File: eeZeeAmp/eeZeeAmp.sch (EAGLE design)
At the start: 11 parts, among them IC1 LM386

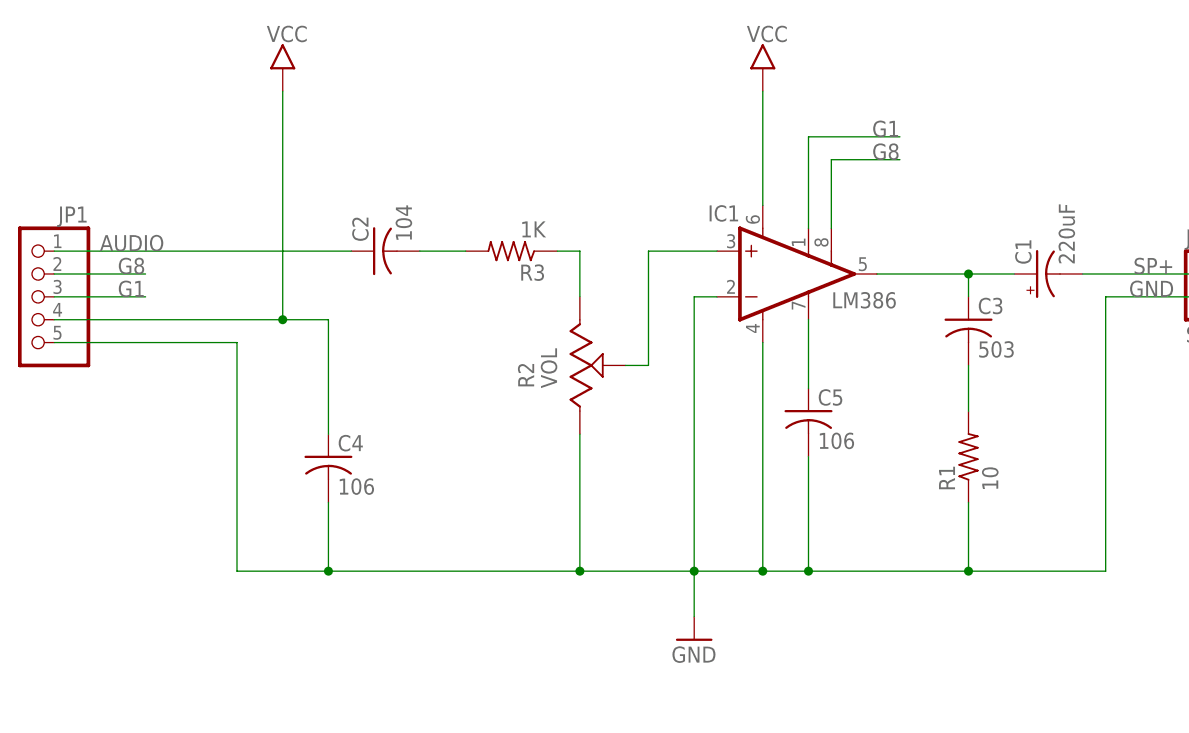
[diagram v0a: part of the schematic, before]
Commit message: Minor updates, added gerbers, zip
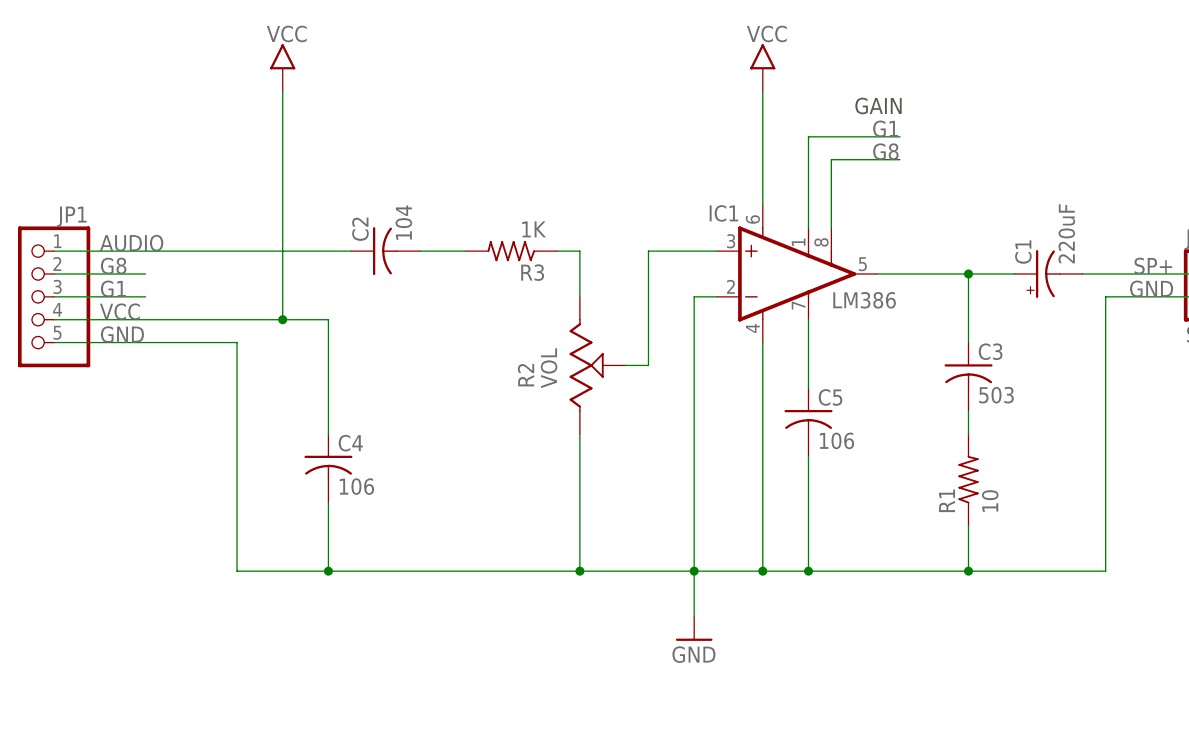
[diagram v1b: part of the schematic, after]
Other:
- note added: "GAIN"
- moved on the sheet: C3, R1
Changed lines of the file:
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@@
 <text x="159.258" y="24.13" size="3.81" layer="94">eeZeeAmp</text>
 <text x="231.14" y="24.13" size="3.81" layer="94">R0.1</text>
+<text x="142.24" y="129.54" size="1.778" layer="97">GAIN</text>
 </plain>
 <instances>
@@
 <instance part="C1" gate="G$1" x="162.56" y="111.76" rot="R90"/>
 <instance part="C2" gate="G$1" x="88.9" y="114.3" rot="R90"/>
-<instance part="C3" gate="G$1" x="154.94" y="106.68"/>
-<instance part="R1" gate="G$1" x="154.94" y="91.44" rot="R90"/>
+<instance part="C3" gate="G$1" x="154.94" y="101.6"/>
+<instance part="R1" gate="G$1" x="154.94" y="88.9" rot="R90"/>
 <instance part="R2" gate="1" x="111.76" y="101.6"/>
 <instance part="JP2" gate="A" x="185.42" y="109.22"/>
@@
 <pinref part="C3" gate="G$1" pin="1"/>
 <wire x1="160.02" y1="111.76" x2="154.94" y2="111.76" width="0.1524" layer="91"/>
-<wire x1="154.94" y1="111.76" x2="154.94" y2="109.22" width="0.1524" layer="91"/>
+<wire x1="154.94" y1="111.76" x2="154.94" y2="104.14" width="0.1524" layer="91"/>
 <junction x="154.94" y="111.76"/>
 <pinref part="IC1" gate="G$1" pin="OUT"/>
@@
 <pinref part="C3" gate="G$1" pin="2"/>
 <pinref part="R1" gate="G$1" pin="2"/>
-<wire x1="154.94" y1="96.52" x2="154.94" y2="101.6" width="0.1524" layer="91"/>
+<wire x1="154.94" y1="93.98" x2="154.94" y2="96.52" width="0.1524" layer="91"/>
 </segment>
 </net>
@@
 <junction x="78.74" y="106.68"/>
 <pinref part="JP1" gate="A" pin="4"/>
+<label x="58.42" y="106.68" size="1.778" layer="95"/>
 </segment>
 </net>
@@
 <wire x1="132.08" y1="78.74" x2="137.16" y2="78.74" width="0.1524" layer="91"/>
 <wire x1="137.16" y1="78.74" x2="154.94" y2="78.74" width="0.1524" layer="91"/>
-<wire x1="154.94" y1="78.74" x2="154.94" y2="86.36" width="0.1524" layer="91"/>
+<wire x1="154.94" y1="78.74" x2="154.94" y2="83.82" width="0.1524" layer="91"/>
 <wire x1="182.88" y1="109.22" x2="170.18" y2="109.22" width="0.1524" layer="91"/>
 <wire x1="170.18" y1="109.22" x2="170.18" y2="78.74" width="0.1524" layer="91"/>
@@
 <junction x="137.16" y="78.74"/>
 <pinref part="JP1" gate="A" pin="5"/>
+<label x="58.42" y="104.14" size="1.778" layer="95"/>
 </segment>
 </net>
@@
 <pinref part="JP1" gate="A" pin="3"/>
 <wire x1="53.34" y1="109.22" x2="63.5" y2="109.22" width="0.1524" layer="91"/>
-<label x="63.5" y="109.22" size="1.778" layer="95" rot="MR0"/>
+<label x="58.42" y="109.22" size="1.778" layer="95"/>
 </segment>
 </net>
@@
 <pinref part="JP1" gate="A" pin="2"/>
 <wire x1="53.34" y1="111.76" x2="63.5" y2="111.76" width="0.1524" layer="91"/>
-<label x="63.5" y="111.76" size="1.778" layer="95" rot="MR0"/>
+<label x="58.42" y="111.76" size="1.778" layer="95"/>
 </segment>
 </net>
